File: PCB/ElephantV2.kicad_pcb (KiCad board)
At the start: 2 copper layers, 128.2 x 77.6 mm, 45 parts, among them U1 Nice_Nano_V2

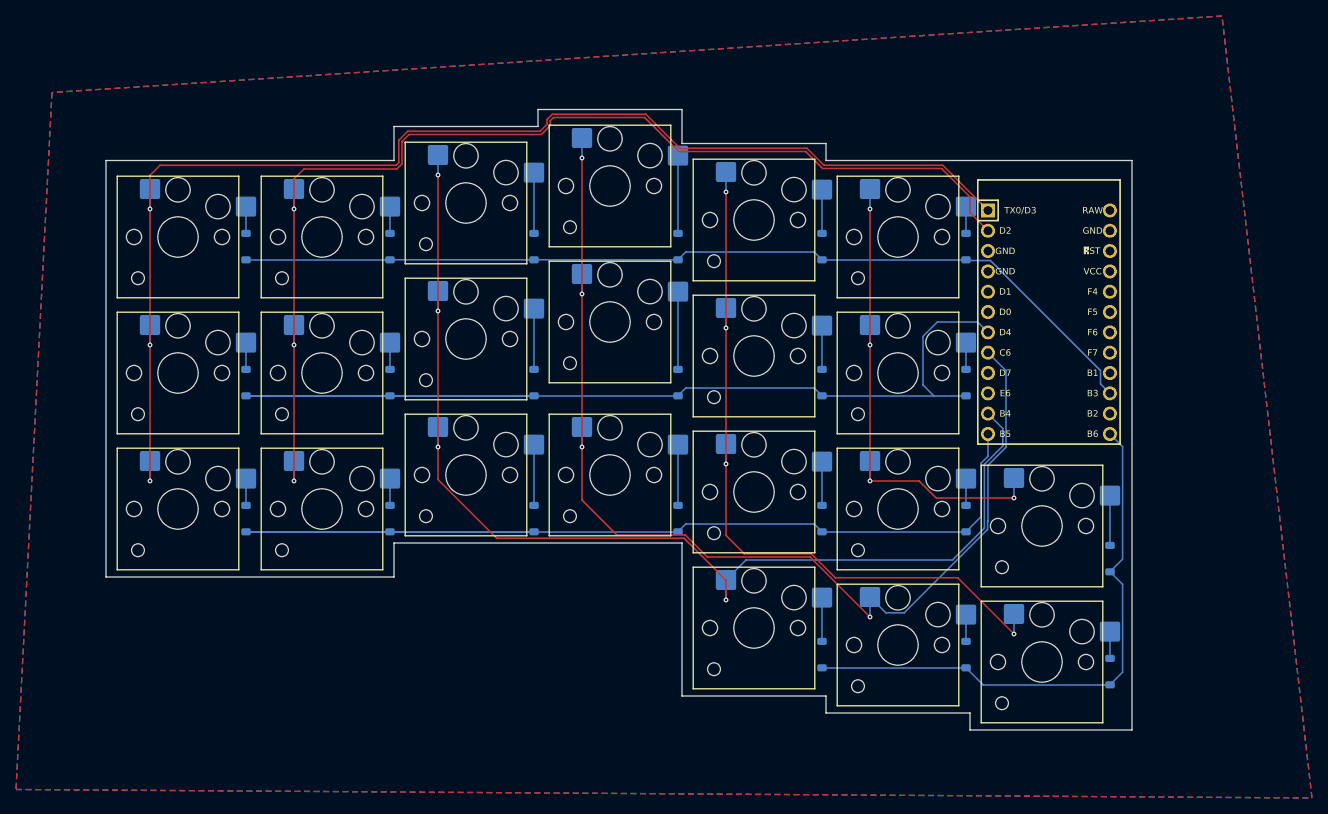
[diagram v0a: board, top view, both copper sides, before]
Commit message: commit
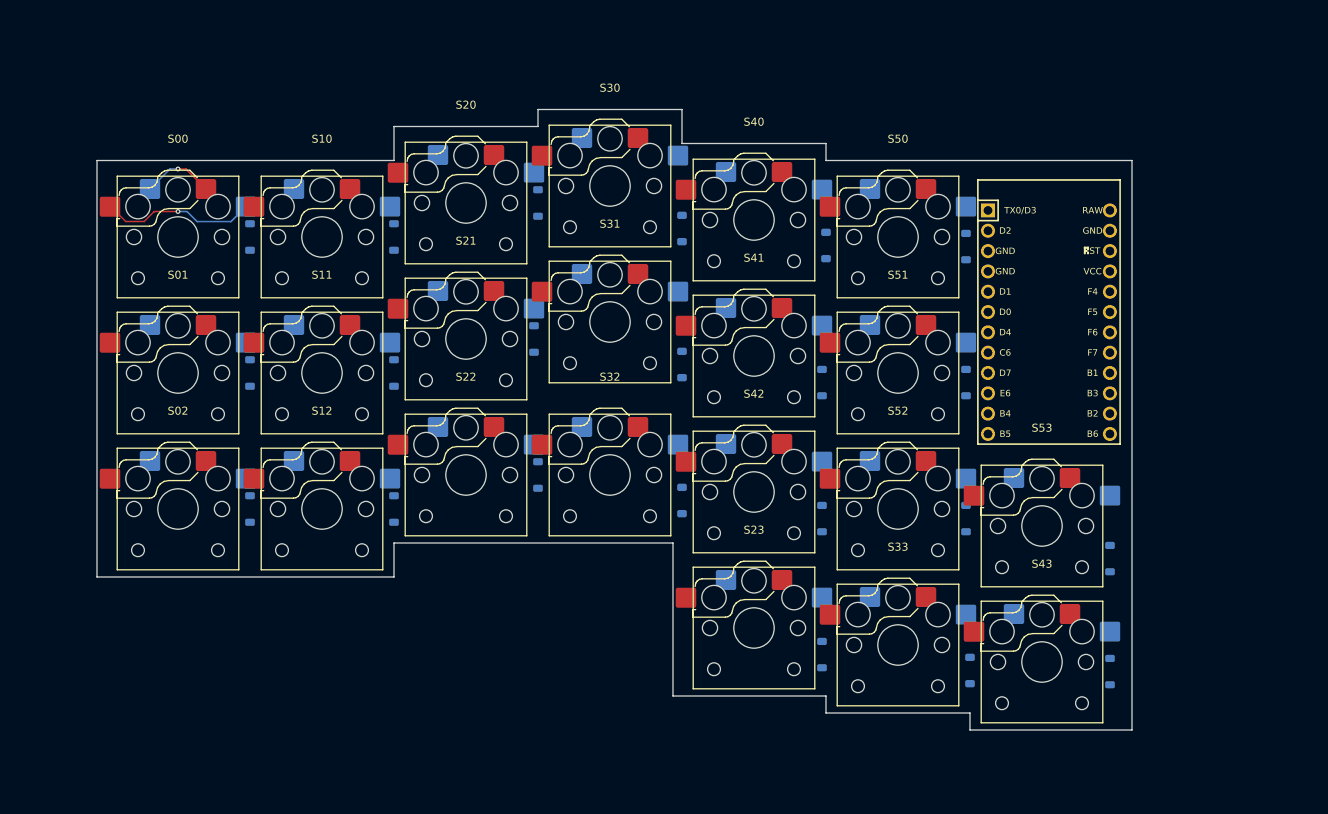
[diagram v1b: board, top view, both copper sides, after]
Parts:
- S00, S01, S02, S10, S11, S12, S20, S21, S22, S23, S30, S31, S32, S33, S40, S41, S42, S43, S50, S51, S52, S53: footprint ScottoKeebs_Hotswap:Hotswap_Choc_V1V2_1.00u -> Reversable_Rok_Prezelj:Choc_1.00u_reversable
- moved D22 5.47 mm to (45.0, 29.8)
- moved D20 5.47 mm to (45.0, -4.25)
- moved D21 5.45 mm to (44.5, 12.8)
- moved D32 2.32 mm to (63.0, 32.9)
- moved D30 2.32 mm to (63.0, -1.06)
- moved D31 2.32 mm to (63.0, 15.9)
- moved D33 2.05 mm to (99.0, 54.2)
- moved D02 1.30 mm to (9.00, 34.0)
- moved D12 1.30 mm to (27.0, 34.0)
- moved D00 1.30 mm to (9.00, 0.00)
- moved D10 1.30 mm to (27.0, 0.00)
- moved D01 1.30 mm to (9.00, 17.0)
- moved D11 1.30 mm to (27.0, 17.0)
- moved D40 0.52 mm to (81.0, 1.06)
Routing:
- net R1: track 162.2 -> 0.00 mm
- net R2: track 158.2 -> 0.00 mm
- net C0: track 160.6 -> 9.07 mm, vias 3 -> 1
- net C1: track 144.2 -> 0.00 mm, vias 3 -> 0
- net C2: track 142.8 -> 0.00 mm, vias 4 -> 0
- net C3: track 138.6 -> 0.00 mm, vias 4 -> 0
- net R0: track 116.7 -> 0.00 mm
- net C4: track 94.0 -> 0.00 mm, vias 4 -> 0
- net R3: track 70.9 -> 0.00 mm
- net C5: track 62.9 -> 0.00 mm, vias 4 -> 0
- net Net-(D00-A): track 3.35 -> 19.5 mm, vias 0 -> 1
- net Net-(D31-A): track 9.73 -> 0.00 mm
- net Net-(D30-A): track 9.73 -> 0.00 mm
- net Net-(D21-A): track 7.60 -> 0.00 mm
- net Net-(D20-A): track 7.60 -> 0.00 mm
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- removed copper zone on B.Cu, net GND
- removed copper zone on F.Cu, net GND
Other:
- board size 128.2 x 77.6 mm -> 129.4 x 77.6 mm
